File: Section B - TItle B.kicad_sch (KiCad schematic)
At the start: 12 parts, among them J2 CE, J3 Conn_01x03_Pin, U2 TLV73333PDBV, U3 MSPM0C1104SDSGR

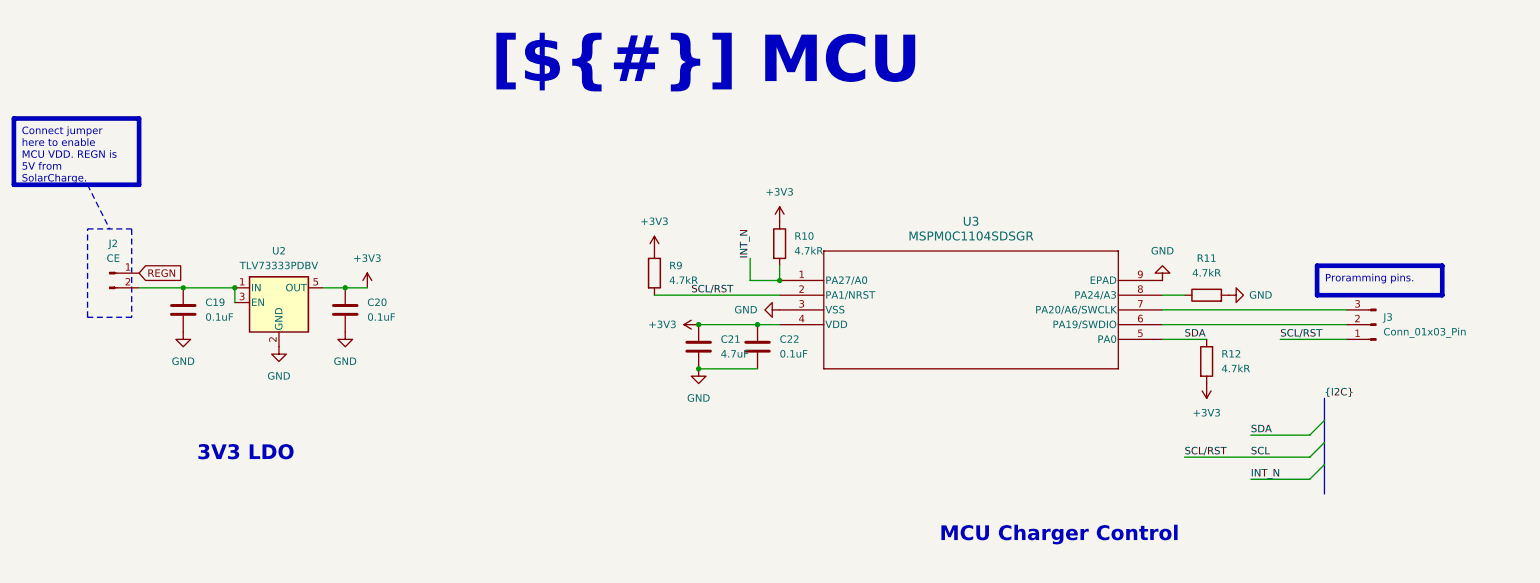
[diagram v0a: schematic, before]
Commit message: First layout
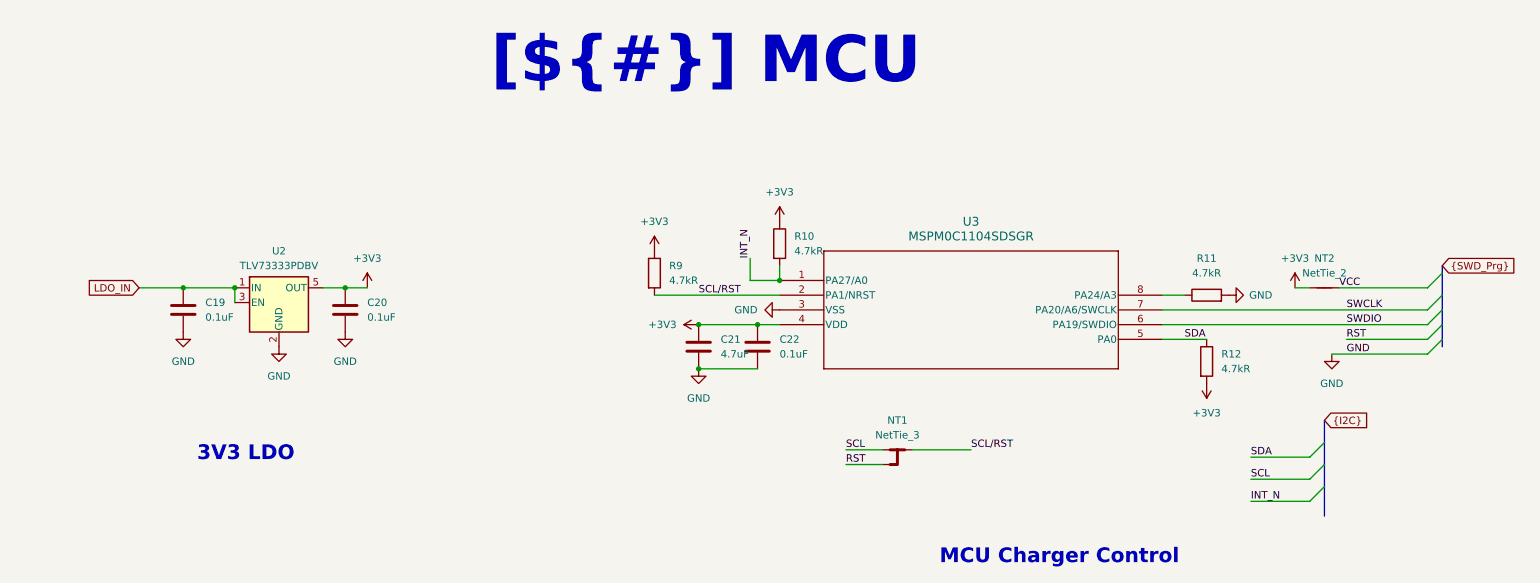
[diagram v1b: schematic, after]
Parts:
- removed J2: CE, Connector_PinHeader_2.54mm:PinHeader_1x02_P2.54mm_Vertical, symbol Connector:Conn_01x02_Pin
- removed J3: Conn_01x03_Pin, Connector_PinSocket_2.54mm:PinSocket_1x03_P2.54mm_Vertical, symbol Connector:Conn_01x03_Pin
- added NT1: NetTie_3, NetTie:NetTie-3_SMD_Pad0.5mm, symbol Device:NetTie_3
- added NT2: NetTie_2, NetTie:NetTie-2_SMD_Pad0.5mm, symbol Device:NetTie_2
- U3: footprint Package_TO_SOT_SMD:TSOT-23-8 -> solar_station:TSOT-23-8-shrink
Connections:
- net +3V3: now also NT2.1
- net GND: no longer U3.9 (EPAD)
- net SCL: now also NT1.1; no longer R9.2, U3.2 (PA1/NRST)
- net LDO_IN: now reaches C19.2, U2.1 (IN), U2.3 (EN)
- net SWDIO: now reaches U3.6 (PA19/SWDIO)
- net SWCLK: now reaches U3.7 (PA20/A6/SWCLK)
- new net RST: NT1.3
- new net SCL/RST: NT1.2, R9.2, U3.2 (PA1/NRST)
- new net VCC: NT2.2
